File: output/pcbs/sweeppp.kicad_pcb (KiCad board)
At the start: 2 copper layers, 136.5 x 111 mm, 61 parts

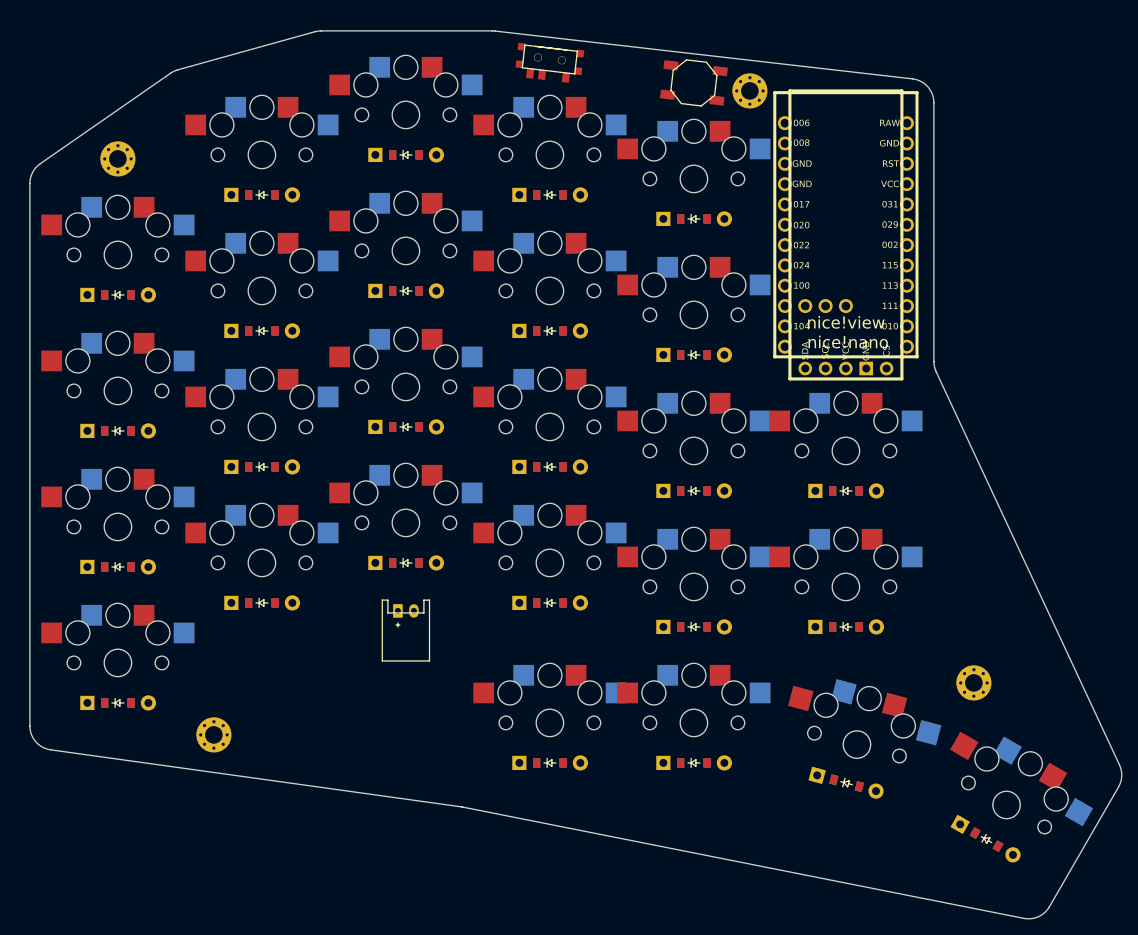
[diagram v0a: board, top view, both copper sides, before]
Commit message: Routed pcb
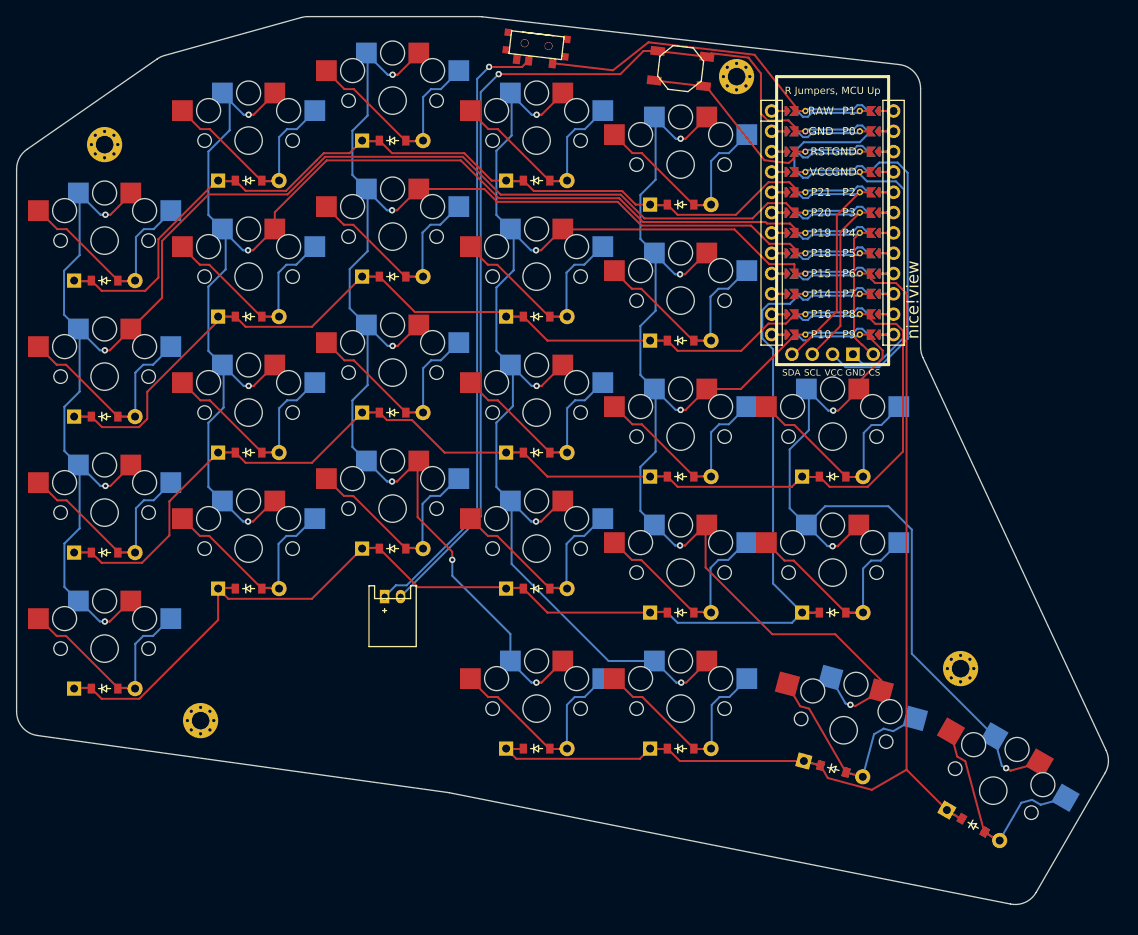
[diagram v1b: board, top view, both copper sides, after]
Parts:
- MCU1: value nice_nano -> (none); footprint nice_nano -> ceoloide:mcu_nice_nano
- moved MCU1 3.25 mm to (189.3, 43.7), turned to 0 degrees
- moved T1 2.44 mm to (152.3, 22.7)
- moved S25 2.44 mm to (190.7, 108.4)
- moved D13 2.44 mm to (152.3, 90.7)
- moved niceView1 2.44 mm to (189.3, 62.7)
- moved S11 2.44 mm to (134.3, 46.7)
- moved _2 2.44 mm to (110.3, 107.2)
- moved D19 2.44 mm to (170.3, 59.7)
- moved D8 2.44 mm to (116.3, 39.7)
- moved _1 2.44 mm to (98.3, 35.2)
- moved D3 2.44 mm to (98.3, 69.2)
- moved D6 2.44 mm to (116.3, 73.7)
- moved S18 2.44 mm to (170.3, 71.7)
- moved S2 2.44 mm to (98.3, 81.2)
- moved S9 2.44 mm to (134.3, 80.7)
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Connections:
- net P006 renamed MCU1_1
- net P008 renamed MCU1_2
- net P029 renamed MCU1_19
- net P031 renamed MCU1_20
- D1 pad 1: P022 -> P7
- D10 pad 1: P024 -> P8
- D11 pad 1: P100 -> P16
- D12 pad 1: P011 -> P21
- D13 pad 1: P022 -> P7
- D14 pad 1: P024 -> P8
- D15 pad 1: P100 -> P16
- D16 pad 1: P011 -> P21
- D17 pad 1: P022 -> P7
- D18 pad 1: P024 -> P8
- D19 pad 1: P100 -> P16
- D2 pad 1: P024 -> P8
- D20 pad 1: P011 -> P21
- D21 pad 1: P022 -> P7
- D22 pad 1: P024 -> P8
- D23 pad 1: P104 -> P6
- D24 pad 1: P104 -> P6
- D25 pad 1: P104 -> P6
- D26 pad 1: P104 -> P6
- D3 pad 1: P100 -> P16
- D4 pad 1: P011 -> P21
- D5 pad 1: P022 -> P7
- D6 pad 1: P024 -> P8
- D7 pad 1: P100 -> P16
- D8 pad 1: P011 -> P21
- D9 pad 1: P022 -> P7
- MCU1 pad 10: P011 -> MCU1_10
- MCU1 pad 11: P104 -> MCU1_11
- MCU1 pad 12: P106 -> MCU1_12
- MCU1 pad 13: P009 -> MCU1_13
- MCU1 pad 14: P010 -> MCU1_14
- MCU1 pad 15: P111 -> MCU1_15
- MCU1 pad 16: P113 -> MCU1_16
- MCU1 pad 17: P115 -> MCU1_17
- MCU1 pad 18: P002 -> MCU1_18
- MCU1 pad 21: VCC -> MCU1_21
- MCU1 pad 22: RST -> MCU1_22
- MCU1 pad 23: GND -> MCU1_23
- MCU1 pad 24: RAW -> MCU1_24
- MCU1 pad 3: GND -> MCU1_3
- MCU1 pad 4: GND -> MCU1_4
- MCU1 pad 5: P017 -> MCU1_5
- MCU1 pad 6: P020 -> MCU1_6
- MCU1 pad 7: P022 -> MCU1_7
- MCU1 pad 8: P024 -> MCU1_8
- MCU1 pad 9: P100 -> MCU1_9
- S1 pad 1: P115 -> P20
- S10 pad 1: P111 -> P18
- S11 pad 1: P111 -> P18
- S12 pad 1: P111 -> P18
- S13 pad 1: P010 -> P15
- S14 pad 1: P010 -> P15
- S15 pad 1: P010 -> P15
- S16 pad 1: P010 -> P15
- S17 pad 1: P009 -> P10
- S18 pad 1: P009 -> P10
- S19 pad 1: P009 -> P10
- S2 pad 1: P115 -> P20
- S20 pad 1: P009 -> P10
- S21 pad 1: P106 -> P9
- S22 pad 1: P106 -> P9
- S23 pad 1: P111 -> P18
- S24 pad 1: P010 -> P15
- S25 pad 1: P009 -> P10
- S26 pad 1: P106 -> P9
- S3 pad 1: P115 -> P20
- S4 pad 1: P115 -> P20
- S5 pad 1: P113 -> P19
- S6 pad 1: P113 -> P19
- S7 pad 1: P113 -> P19
- S8 pad 1: P113 -> P19
- S9 pad 1: P111 -> P18
- niceView1 pad 1: P002 -> P4
- niceView1 pad 4: P020 -> P3
- niceView1 pad 5: P017 -> P2
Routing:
- net P20: track 0.00 -> 201.3 mm, vias 0 -> 4
- net P18: track 0.00 -> 192.4 mm, vias 0 -> 6
- net GND: track 0.00 -> 192.0 mm, vias 0 -> 1
- net P7: track 0.00 -> 179.3 mm
- net P19: track 0.00 -> 175.2 mm, vias 0 -> 4
- net P15: track 0.00 -> 172.4 mm, vias 0 -> 5
- net P8: track 0.00 -> 165.3 mm
- net P10: track 0.00 -> 157.9 mm, vias 0 -> 5
- net P6: track 0.00 -> 148.9 mm
- net P21: track 0.00 -> 129.4 mm
- net P16: track 0.00 -> 128.2 mm
- net P9: track 0.00 -> 109.2 mm, vias 0 -> 3
- net BAT: track 0.00 -> 77.7 mm, vias 0 -> 1
- net VCC: track 0.00 -> 47.8 mm
- net RAW: track 0.00 -> 45.2 mm
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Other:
- net class Default removed
